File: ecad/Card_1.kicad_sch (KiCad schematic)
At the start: 61 parts, among them J3 Conn_01x03_Pin, J4 USB_C_Receptacle_USB2.0_14P, SW15 SW_Push, SW16 SW_Push, U10 MCP23017_SO, U11 NCP1117-3.3_SOT223, U6 MCP23017_SO, U8 W25Q128JVS, U9 RP2350_80QFN, X2 ABM8-272-T3

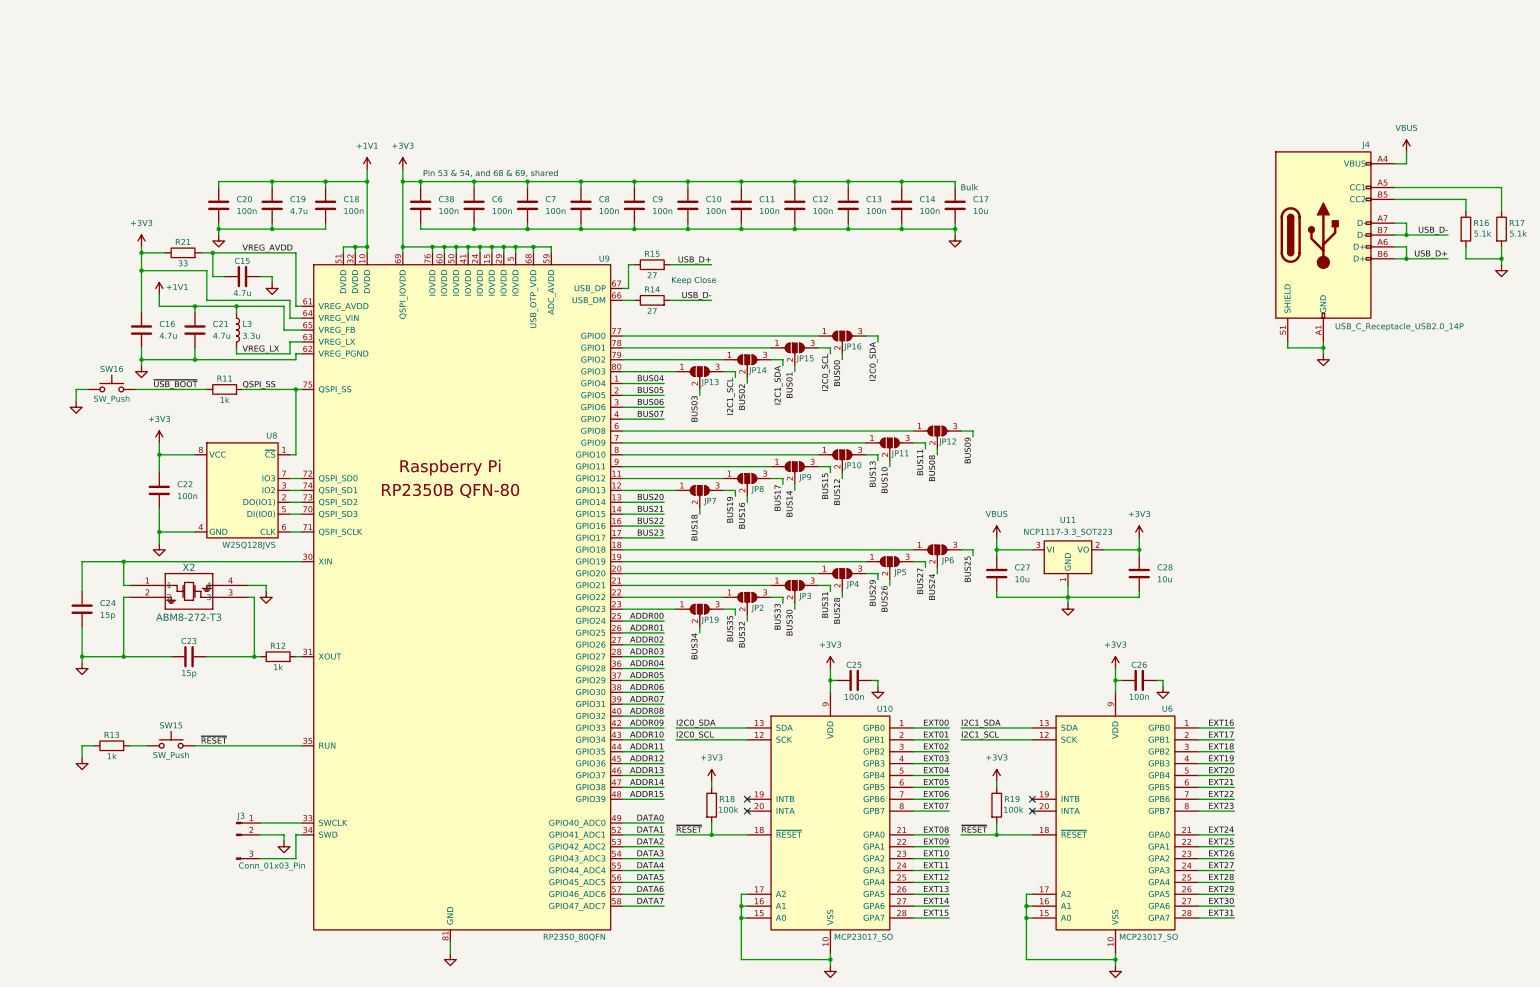
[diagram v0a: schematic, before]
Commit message: new card boxes
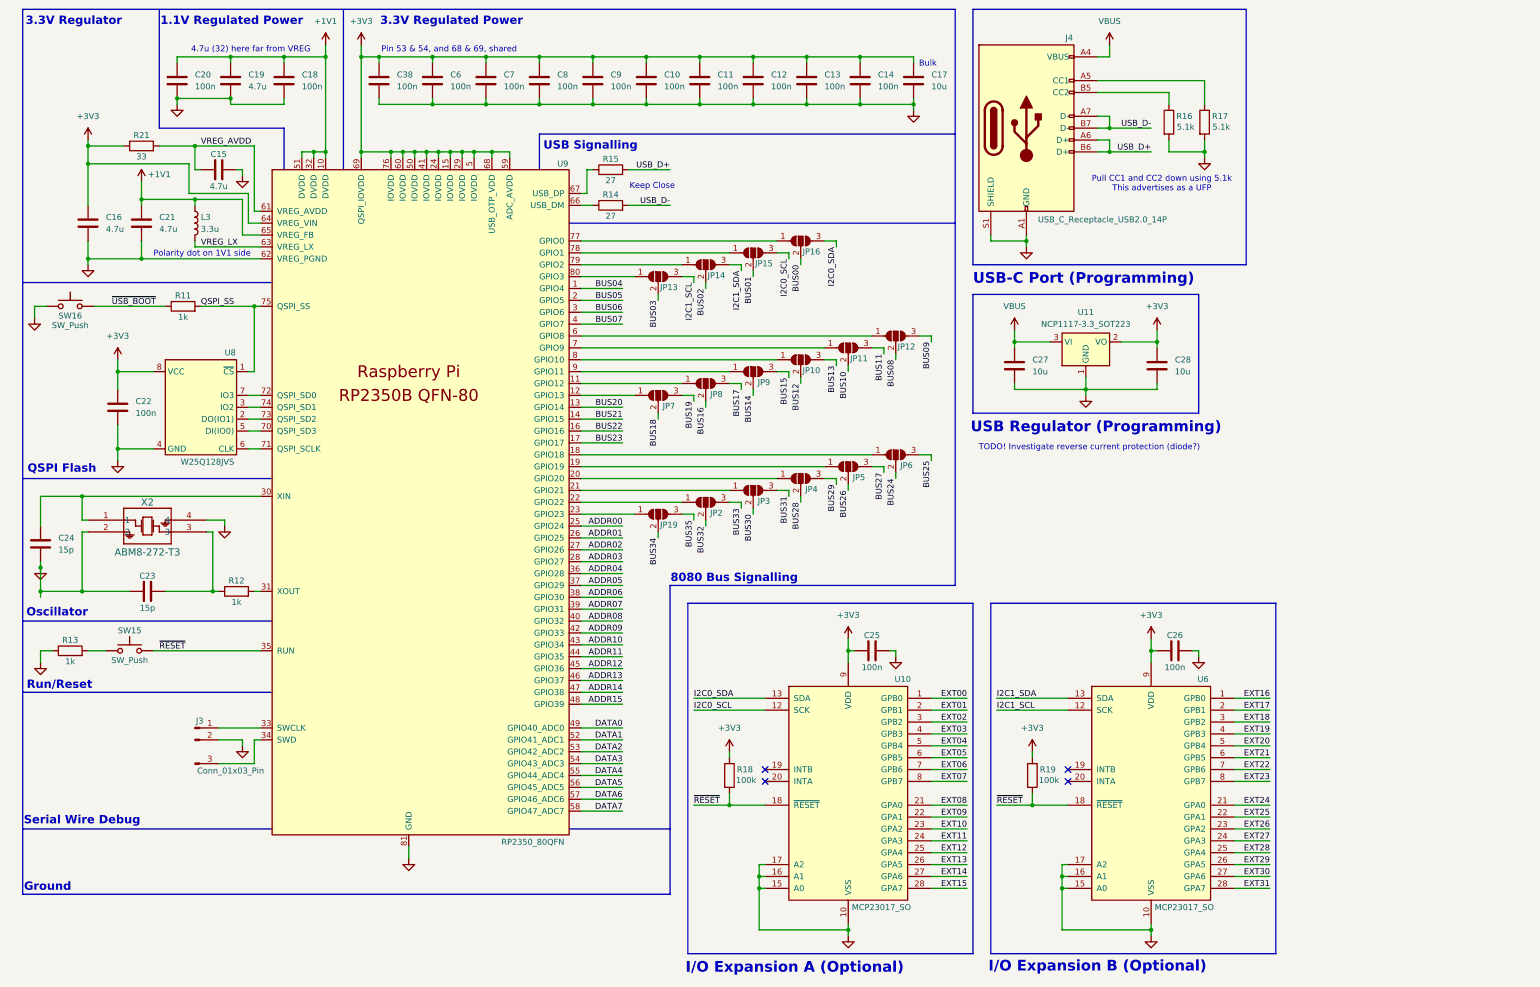
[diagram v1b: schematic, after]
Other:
- note added: "1.1V Regulated Power"
- note added: "3.3V Regulated Power"
- note added: "3.3V Regulator"
- note added: "4.7u (32) here far from VREG"
- note added: "8080 Bus Signalling"
- note added: "Ground"
- note added: "I/O Expansion A (Optional)"
- note added: "I/O Expansion B (Optional)"
- note added: "Oscillator"
- note added: "Polarity dot on 1V1 side"
- note added: "Pull CC1 and CC2 down using 5.1k This advertises as a UFP"
- note added: "QSPI Flash"
- note added: "Run/Reset"
- note added: "Serial Wire Debug"
- note added: "TODO! Investigate reverse current protection (diode?)"
- note added: "USB Regulator (Programming)"
- note added: "USB Signalling"
- note added: "USB-C Port (Programming)"
- title: CPU Card for Miniaturized Altair 8800  -> Generic Card for Miniaturized Altair 8800 
- moved on the sheet: C10, C11, C12, C13, C14, C15, C16, C17, C18, C19, C20, C21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
